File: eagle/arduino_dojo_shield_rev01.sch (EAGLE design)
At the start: 26 parts, among them IC1 74LS595N, J1 ARDUINO_R3_SHIELDNOLABELS, M1 SMALL_SERVO, M2 SMALL_SERVO

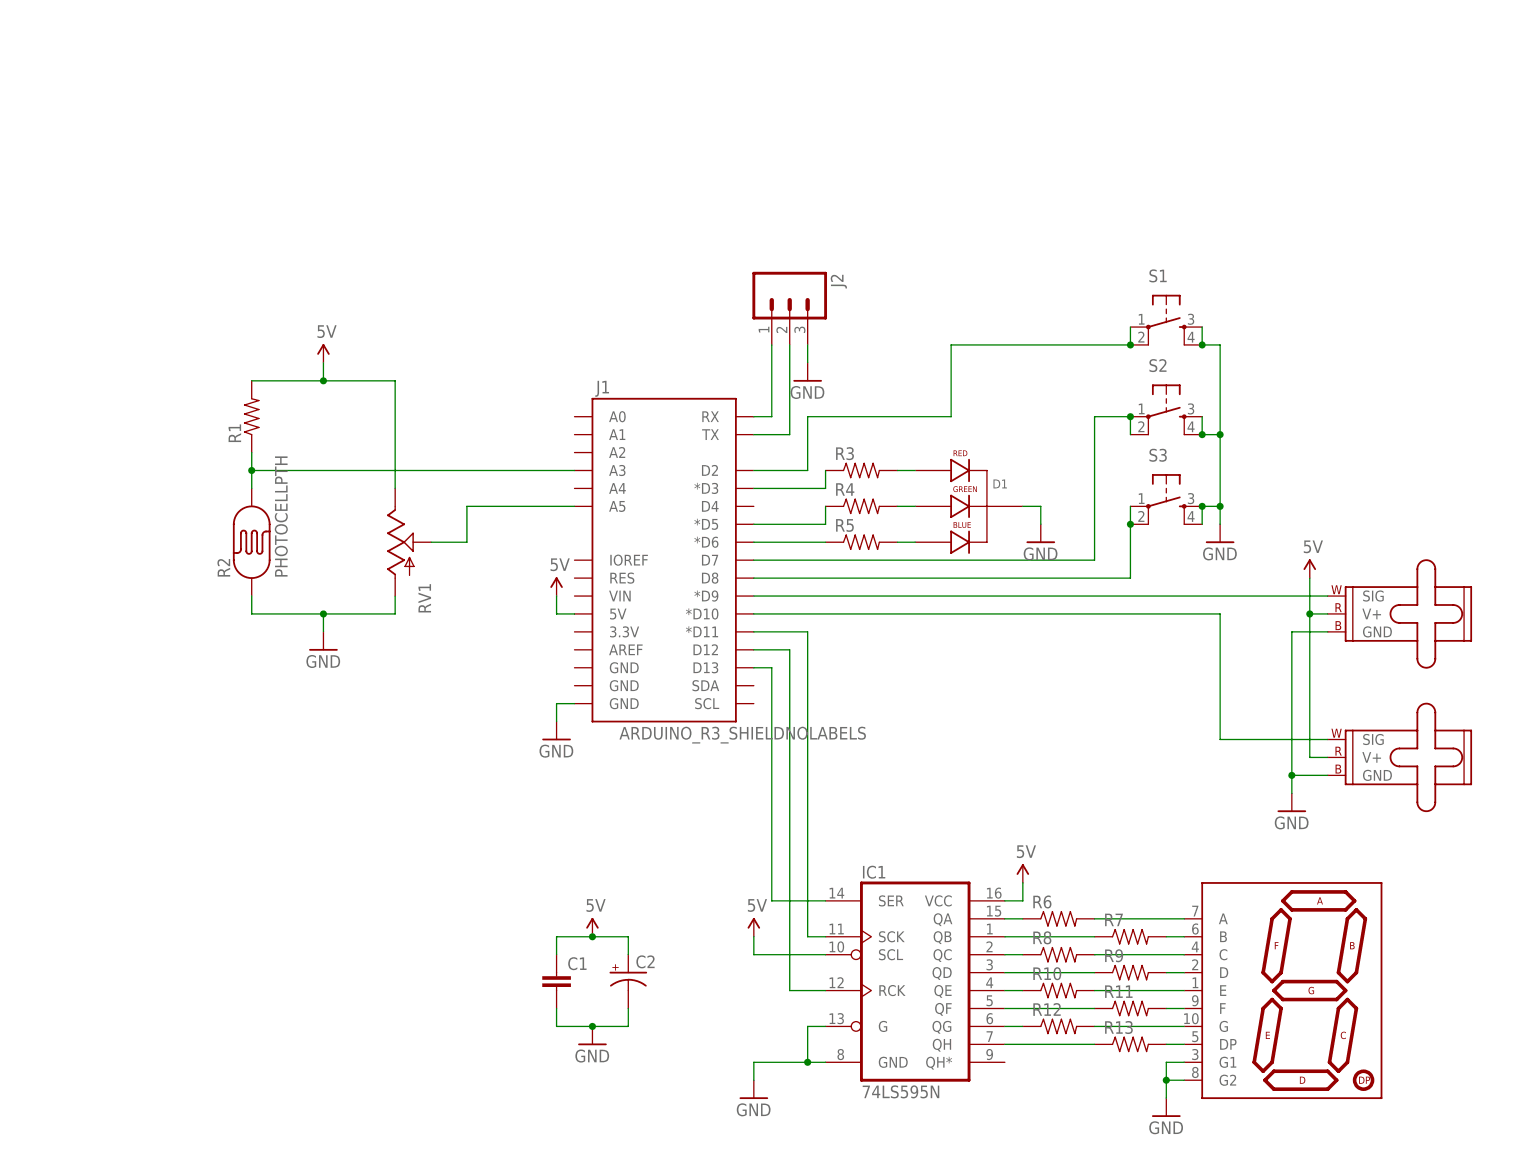
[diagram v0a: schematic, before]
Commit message: rev 01 - sem layout
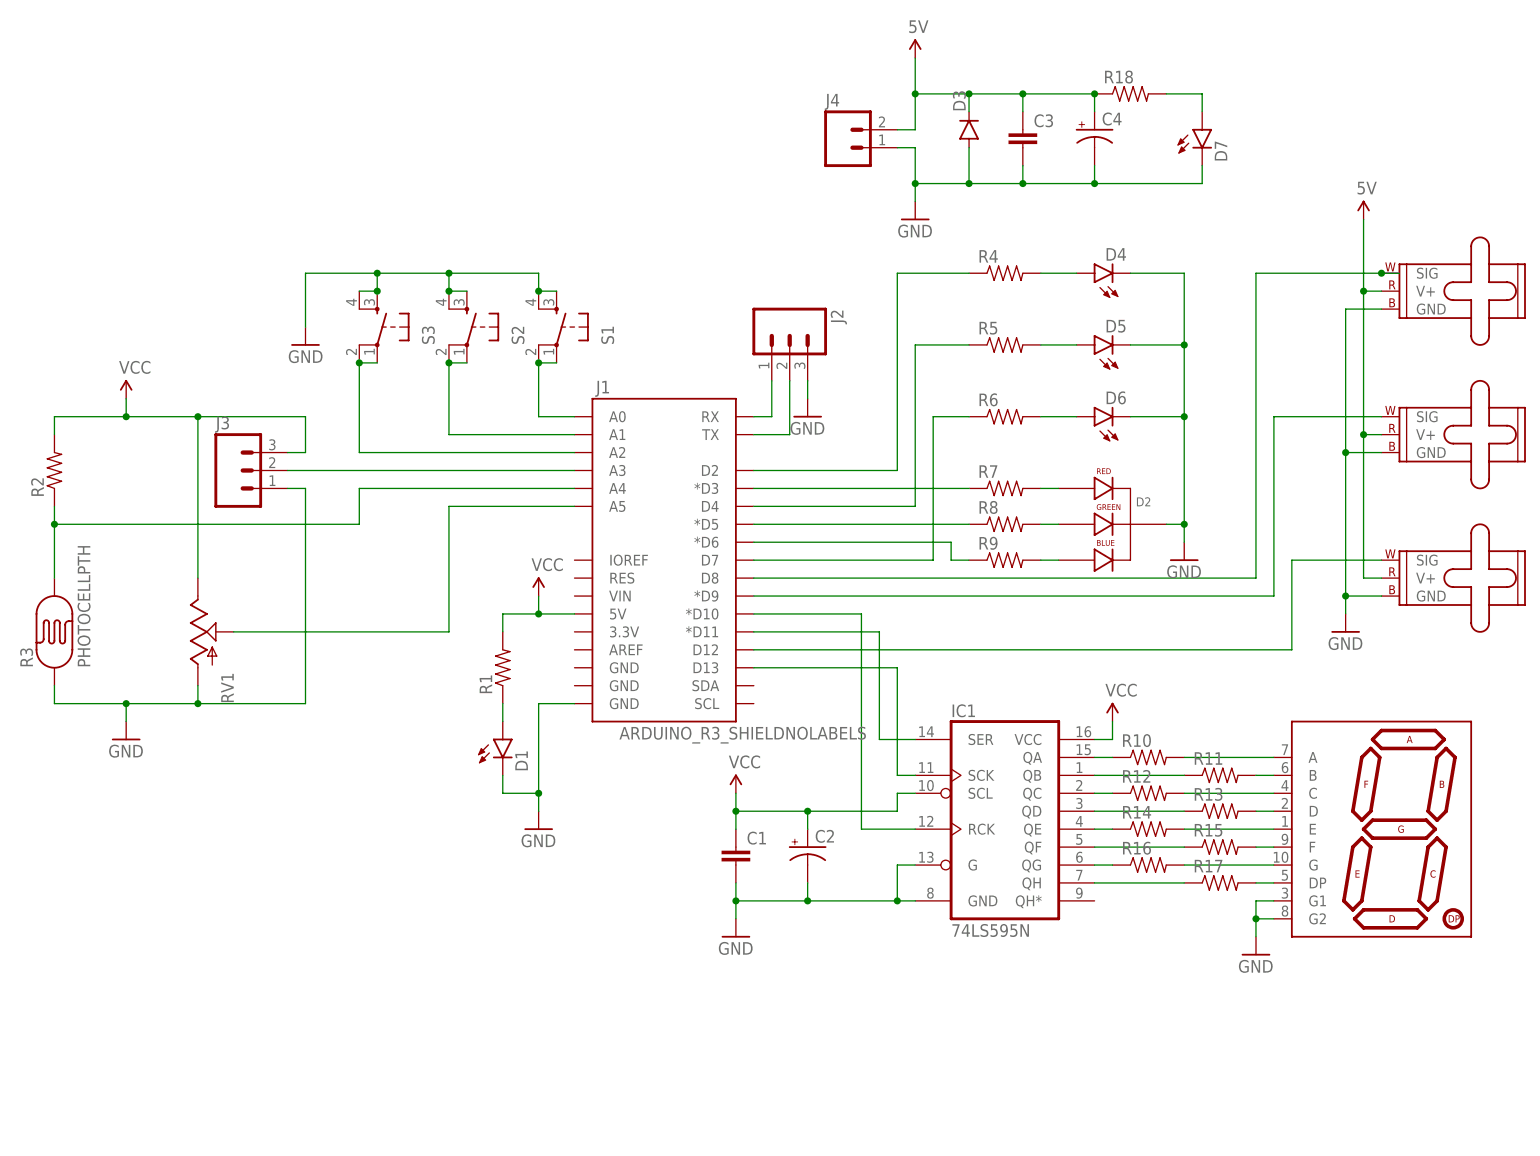
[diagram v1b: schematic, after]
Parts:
- added C3: (no value), SparkFun-Capacitors:0.1UF-50V-20%(PTH)KIT-EZ
- added C4: (no value), SparkFun-Capacitors:10UF-25V-20%(PTH)
- added D2: LED-RGB-CC-THRUCLEAR, SparkFun-LED:LED-RGB-CC-THRUCLEAR
- added D3: (no value), SparkFun-DiscreteSemi:DIODEKIT
- added D4, D5, D6, D7: (no value), SparkFun-LED:LED3MM
- added J3: (no value), SparkFun-Connectors:M03PTH
- added J4: (no value), SparkFun-Connectors:M025MM
- added M3: SMALL_SERVO, GH_SparkFun-Electromechanical:SMALL_SERVO
- added R14, R15, R16, R17, R18: (no value), SparkFun-Passives:RESISTOR0805-RES
- D1: value LED-RGB-CC-THRUCLEAR -> (none); device SparkFun-LED:LED-RGB-CC-THRUCLEAR -> SparkFun-LED:LED3MM
- J1: device SparkFun-Boards:ARDUINO_R3_SHIELDNOLABELS -> GH_SparkFun-Boards:ARDUINO_R3_SHIELDNOLABELS
- M1, M2: device SparkFun-Electromechanical:SMALL_SERVO -> GH_SparkFun-Electromechanical:SMALL_SERVO
- R1: device SparkFun-Passives:RESISTORPTH-1/4W -> SparkFun-Passives:RESISTOR0805-RES
- R2: value PHOTOCELLPTH -> (none); device SparkFun-Sensors:PHOTOCELLPTH -> SparkFun-Passives:RESISTORPTH-1/4W
- R3: value (none) -> PHOTOCELLPTH; device SparkFun-Passives:RESISTOR0805-RES -> SparkFun-Sensors:PHOTOCELLPTH
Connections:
- removed net N$17 (its old number): J1.*D10, M2.SIG
- removed net N$34: IC1.RCK, J1.D12
- new net N$16: J1.D12, M2.SIG
- new net N$2: J1.A3, J3.2
- new net N$24: IC1.SER, J1.*D11
- new net N$32: J1.D8, M3.SIG
- new net N$37: J1.A0, S1.1, S1.2
- new net N$38: D1.A, R1.1
- new net N$40: D5.A, R5.2
- new net N$41: D6.A, R6.2
- new net N$42: D4.A, R4.2
- new net N$43: J1.D4, R5.1
- new net N$44: J1.D2, R4.1
- new net N$45: IC1.RCK, J1.*D10
- new net VCC: C1.1, C2.+, IC1.SCL, IC1.VCC, J1.5V, J3.3, R1.2, R2.2, RV1.E
- net 5V: now also C3.1, C4.+, D3.C, J4.2, M3.V+, R18.1; no longer C1.1, C2.+, IC1.SCL, IC1.VCC, J1.5V, R1.2, RV1.E
- net GND: now also C3.2, C4.-, D1.C, D2.CATHODE, D3.A, D4.C, D5.C, D6.C, D7.C, J3.1, J4.1, M3.GND, R3.P$1; no longer D1.CATHODE, R2.P$1
- net N$1: now also J1.A4, R2.1, R3.P$2; no longer J1.A3, R1.1, R2.P$2
- net N$10: now also D2.GREEN_CATHODE, R8.2; no longer D1.GREEN_CATHODE, R4.2
- net N$11: now also D2.BLUE_CATHODE, R9.2; no longer D1.BLUE_CATHODE, R5.2
- net N$12: now also R6.1; no longer S2.1, S2.2
- net N$13: now also IC1.SCK, J1.D13; no longer J1.D8, S3.1, S3.2
- net N$14: now also R10.1; no longer R6.1
- net N$15: now also R10.2; no longer R6.2
- net N$18: now also R11.1; no longer R7.1
- net N$19: now also R11.2; no longer R7.2
- net N$20: now also R12.1; no longer R8.1
- net N$21: now also R12.2; no longer R8.2
- net N$22: now also R13.1; no longer R9.1
- net N$23: now also R13.2; no longer R9.2
- net N$25: now also R14.2; no longer R10.2
- net N$26: now also R15.1; no longer R11.1
- net N$27: now also R15.2; no longer R11.2
- net N$28: now also R16.1; no longer R12.1
- net N$29: now also R16.2; no longer R12.2
- net N$3: now also R14.1; no longer R10.1
- net N$30: now also R17.1; no longer R13.1
- net N$31: now also R17.2; no longer R13.2
- net N$33: now also D7.A, R18.2; no longer IC1.SER, J1.D13
- net N$35: now also J1.A1, S2.1, S2.2; no longer IC1.SCK, J1.*D11
- net N$36: now also J1.A2, S3.1, S3.2; no longer J1.D2, S1.1, S1.2
- net N$4: now also R9.1; no longer R5.1
- net N$5: now also R8.1; no longer R4.1
- net N$8: now also R7.1; no longer R3.1
- net N$9: now also D2.RED_CATHODE, R7.2; no longer D1.RED_CATHODE, R3.2
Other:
- moved on the sheet: C1, C2, IC1, J2, R1, R10, R11, R12, R13, R4, R5, R6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
